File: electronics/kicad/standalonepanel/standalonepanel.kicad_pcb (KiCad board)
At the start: 2 copper layers, 135 x 54 mm, 87 parts, among them J1 Speaker, J2 POWER, P1 USB-C, P2 USB-A, SW1 TST-ESP32, SW2 BOOT, SW3 TST-ICE40, SW4 RESET, U1 SC189ZSKTRT, U10 MPU-6050, U2 SC189CSKTRT, U3 ESP32-WROVER-E, U4 CH340C, U5 MAX3421E, U6 IS64WV25616EFBLL-10TLI, U7 ICE40-HX4K, U8 DS3231, U9 MAX98357A, X2 12MHz

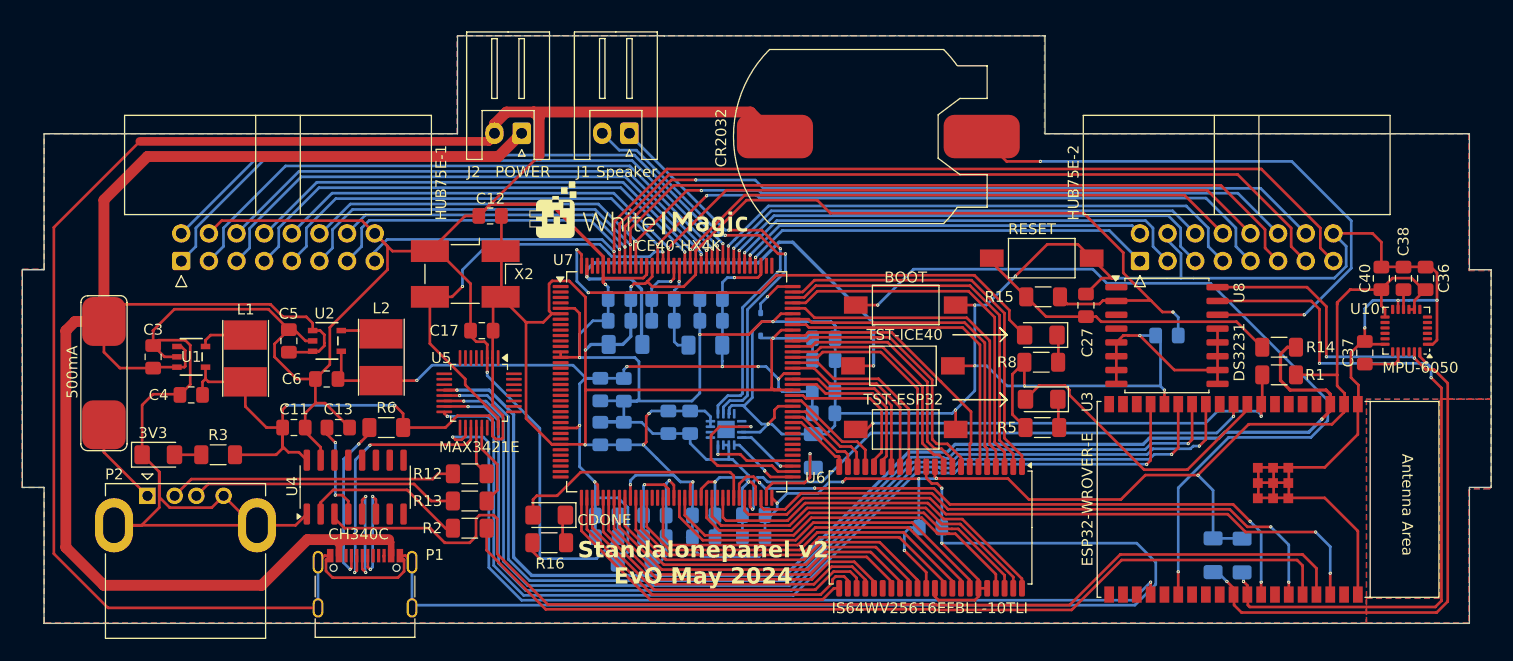
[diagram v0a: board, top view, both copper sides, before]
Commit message: Schematic v2 PCB version v2 send for production
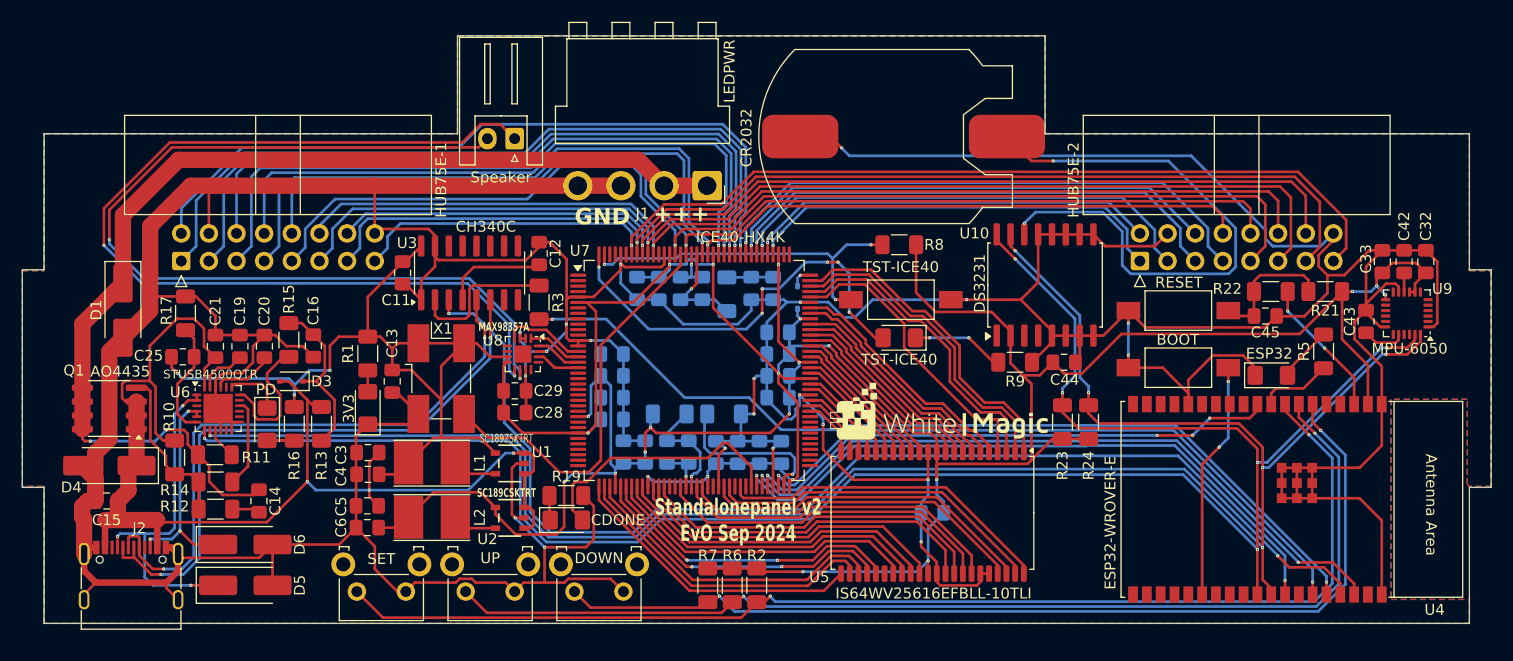
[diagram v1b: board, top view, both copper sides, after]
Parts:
- removed F1: 500mA, 0_project:FUSEHOLDER 1808
- removed P1: USB-C, 0_project:USB_C_Receptacle_G-Switch_GT-USB-7010ASV
- removed P2: USB-A, 0_project:USB-A TH Female
- removed X2: 12MHz, 0_project:Oscillator_SMD_EuroQuartz_XO91-4Pin_7.0x5.0mm_HandSoldering
- added C39: 100nF, Capacitor_SMD:C_0805_2012Metric_Pad1.18x1.45mm_HandSolder, B.Cu at (101.2, 128.2)
- added C41: 4.7uF, Capacitor_SMD:C_0805_2012Metric_Pad1.18x1.45mm_HandSolder, B.Cu at (105.2, 128.2)
- added C42: 100nF, Capacitor_SMD:C_0805_2012Metric_Pad1.18x1.45mm_HandSolder, F.Cu at (171.0, 110.8)
- added C43: 2.2nF/50V, Capacitor_SMD:C_0805_2012Metric_Pad1.18x1.45mm_HandSolder, F.Cu at (167.5, 116.2)
- added C44: 100nF, Capacitor_SMD:C_0805_2012Metric_Pad1.18x1.45mm_HandSolder, F.Cu at (139.8, 120.0)
- added C45: 100nF, Capacitor_SMD:C_0805_2012Metric_Pad1.18x1.45mm_HandSolder, F.Cu at (158.2, 115.8)
- added D1: P4SMA27A, Diode_SMD:D_SMA_Handsoldering, F.Cu at (53.2, 115.2)
- added D3: BAT760, Diode_SMD:D_SOD-323, F.Cu at (68.8, 121.8)
- added D4: P4SMA27A, Diode_SMD:D_SMA_Handsoldering, F.Cu at (52.0, 129.5)
- added D5: P4SMA27A, Diode_SMD:D_SMA_Handsoldering, F.Cu at (64.5, 140.5)
- added D6: P4SMA27A, Diode_SMD:D_SMA_Handsoldering, F.Cu at (64.5, 136.8)
- added J3: Speaker, Connector_JST:JST_XH_S2B-XH-A_1x02_P2.50mm_Horizontal, F.Cu at (89.2, 99.5)
- added LED5: CDONE, LED_SMD:LED_1206_3216Metric_Pad1.42x1.75mm_HandSolder, F.Cu at (94.0, 134.5)
- added Q1: AO4435, Package_SO:SOIC-8_3.9x4.9mm_P1.27mm, F.Cu at (52.0, 124.2)
- added R18: 10K, Resistor_SMD:R_1206_3216Metric_Pad1.30x1.75mm_HandSolder, B.Cu at (108.5, 124.8)
- added R19: 22R, Resistor_SMD:R_1206_3216Metric_Pad1.30x1.75mm_HandSolder, F.Cu at (94.0, 132.2)
- added R20: 100R, Resistor_SMD:R_1206_3216Metric_Pad1.30x1.75mm_HandSolder, B.Cu at (103.5, 124.8)
- added R21: 10K, Resistor_SMD:R_1206_3216Metric_Pad1.30x1.75mm_HandSolder, F.Cu at (163.8, 113.5)
- added R22: 100R, Resistor_SMD:R_1206_3216Metric_Pad1.30x1.75mm_HandSolder, F.Cu at (158.8, 113.5)
- added R23: 2K7, Resistor_SMD:R_1206_3216Metric_Pad1.30x1.75mm_HandSolder, F.Cu at (139.6, 125.5)
- added R24: 2K7, Resistor_SMD:R_1206_3216Metric_Pad1.30x1.75mm_HandSolder, F.Cu at (142.0, 125.5)
- added SW5: TST-ICE40, Button_Switch_SMD:SW_SPST_FSMSM, F.Cu at (124.8, 114.2)
- added SW6: RESET, Button_Switch_SMD:SW_SPST_FSMSM, F.Cu at (150.2, 115.2)
- added X1: 12MHz, 0_project:Oscillator_SMD_EuroQuartz_XO91-4Pin_7.0x5.0mm_HandSoldering, F.Cu at (82.5, 121.5)
- C14, C25, C29, C33, R7: moved to F.Cu
- C15, C20: value 100nF -> 1uF; moved to F.Cu
- C16, C19, C21: value 4.7uF -> 1uF; moved to F.Cu
- C17: value 1uF -> 100nF; moved to B.Cu
- C18, C31, C34: value 100nF -> 4.7uF
- C23: value 10uF -> 4.7uF
- C27, C40: moved to B.Cu
- C28: value 4.7uF -> 10uF; moved to F.Cu
- C30, C35: value 4.7uF -> 100nF
- C32: value 4.7uF -> 10nF; moved to F.Cu
- C36: value 10nF -> 4.7uF; moved to B.Cu
- C37: value 2.2nF/50V -> 100nF; moved to B.Cu
- C38: value 100nF -> 4.7uF; moved to B.Cu
- J1: value Speaker -> LEDPWR; footprint Connector_JST:JST_XH_S2B-XH-A_1x02_P2.50mm_Horizontal -> 0_project:JST_VH_1x04_P3.96mm_Horizontal
- J2: value POWER -> USB_C-PD; footprint Connector_JST:JST_XH_S2B-XH-A_1x02_P2.50mm_Horizontal -> 0_project:USB_C_Receptacle_G-Switch_GT-USB-7010ASV
- LED1: value ESP32 -> 3V3
- LED2: value 3V3 -> ESP32
- LED4: value CDONE -> PD
- R1: value 10K -> 1K5
- R10: value 2K7 -> 100K; moved to F.Cu
- R11: value 2K7 -> 1K; moved to F.Cu
- R12: value 33R -> 100R
- R13: value 33R -> 470R
- R14: value 100R -> 22K
- R15: value 10K -> 1K
- R16: value 22R -> 1K5
- R17: value 100R -> 10K; moved to F.Cu
- R2: value 47R -> 10K
- R3: value 1K5 -> 47R
- R6: value 5K1 -> 10K
- R8: value 2K2 -> 10K
- R9: value 10K -> 2K2; moved to F.Cu
- SW1: value TST-ESP32 -> SET; footprint Button_Switch_SMD:SW_SPST_FSMSM -> 0_project:SW_Tactile_SKHH_Angled
- SW3: value TST-ICE40 -> UP; footprint Button_Switch_SMD:SW_SPST_FSMSM -> 0_project:SW_Tactile_SKHH_Angled
- SW4: value RESET -> DOWN; footprint Button_Switch_SMD:SW_SPST_FSMSM -> 0_project:SW_Tactile_SKHH_Angled
- U10: value MPU-6050 -> DS3231; footprint 0_project:InvenSense_QFN-24_4x4mm_P0.5mm -> Package_SO:SOIC-16W_7.5x10.3mm_P1.27mm
- U3: value ESP32-WROVER-E -> CH340C; footprint 0_project:ESP32-WROVER-E -> Package_SO:SOIC-16_3.9x9.9mm_P1.27mm
- U4: value CH340C -> ESP32-WROVER-E; footprint Package_SO:SOIC-16_3.9x9.9mm_P1.27mm -> 0_project:ESP32-WROVER-E
- U5: value MAX3421E -> IS64WV25616EFBLL-10TLI; footprint 0_project:PQFP-32_5x5mm_P0.5mm -> Package_SO:TSOP-II-44_10.16x18.41mm_P0.8mm
- U6: value IS64WV25616EFBLL-10TLI -> STUSB4500QTR; footprint Package_SO:TSOP-II-44_10.16x18.41mm_P0.8mm -> 0_project:QFN-24-1EP_4x4mm_P0.5mm_EP2.7x2.7mm
- U8: value DS3231 -> MAX98357A; footprint Package_SO:SOIC-16W_7.5x10.3mm_P1.27mm -> Package_DFN_QFN:TQFN-16-1EP_3x3mm_P0.5mm_EP1.6x1.6mm
- U9: value MAX98357A -> MPU-6050; footprint Package_DFN_QFN:TQFN-16-1EP_3x3mm_P0.5mm_EP1.6x1.6mm -> 0_project:InvenSense_QFN-24_4x4mm_P0.5mm; moved to F.Cu
- moved LED2 102.6 mm to (158.8, 121.2)
- moved R14 98.5 mm to (61.8, 131.0), turned to 0 degrees
- moved R10 95.9 mm to (58.0, 128.8)
- moved R11 94.9 mm to (61.7, 128.5), turned to 0 degrees
- moved U4 86.1 mm to (160.7, 132.6), turned to -90 degrees
- moved C14 84.8 mm to (65.8, 132.8), turned to -90 degrees
- moved R1 83.8 mm to (75.8, 119.2), turned to 90 degrees
- moved U3 76.3 mm to (85.1, 111.8), turned to 90 degrees
- moved C38 73.4 mm to (99.2, 128.2)
- moved C32 70.4 mm to (173.0, 110.8), turned to -90 degrees
- moved R15 69.4 mm to (68.5, 117.9), turned to -90 degrees
- moved C40 67.6 mm to (103.2, 128.2)
- moved C33 67.3 mm to (169.0, 110.8), turned to -90 degrees
- moved C15 67.2 mm to (51.8, 132.8), turned to 180 degrees
- moved U6 66.4 mm to (62.0, 124.2), turned to 0 degrees
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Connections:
- C12 pad 1: +3V3 -> Net-(U3-V3)
- C13 pad 1: Net-(U4-V3) -> +3V3
- C14 pad 1: GND -> VPANEL
- C14 pad 2: +3V3 -> Net-(C14-Pad2)
- C15 pad 1: +3V3 -> VBUS
- C16 pad 1: +3V3 -> Net-(D3-K)
- C17 pad 1: GND -> +3V3
- C17 pad 2: +3V3 -> GND
- C18 pad 1: +1V2 -> +3V3
- C19 pad 1: +1V2 -> Net-(U6-VREG_2V7)
- C20 pad 1: +3V3 -> Net-(U6-VREG_1V2)
- C21 pad 1: GND -> VBUS
- C21 pad 2: +1V2 -> GND
- C22 pad 1: GND -> +1V2
- C22 pad 2: +1V2 -> GND
- C23 pad 1: +3V3 -> +1V2
- C25 pad 2: GND -> Net-(U6-RESET)
- C26 pad 1: +3V3 -> GND
- C26 pad 2: GND -> +1V2
- C27 pad 1: Net-(C27-Pad1) -> GND
- C27 pad 2: GND -> +1V2
- C28 pad 1: GND -> +3V3
- C28 pad 2: +1V2 -> GND
- C29 pad 1: GND -> +3V3
- C29 pad 2: +1V2 -> GND
- C3 pad 1: +5V -> VBUS
- C30 pad 1: GND -> +3V3
- C30 pad 2: +3V3 -> GND
- C31 pad 1: GND -> +3V3
- C31 pad 2: +3V3 -> GND
- C34 pad 1: Net-(U7-VCCPLL0) -> GND
- C34 pad 2: Net-(U7-GNDPLL0) -> +3V3
- C35 pad 1: Net-(U7-VCCPLL0) -> GND
- C35 pad 2: Net-(U7-GNDPLL0) -> +3V3
- C37 pad 2: Net-(U10-CPOUT) -> +3V3
- C38 pad 2: Net-(U10-REGOUT) -> +1V2
- C40 pad 1: GND -> Net-(U7-VCCPLL0)
- C40 pad 2: +3V3 -> Net-(U7-GNDPLL0)
- C5 pad 1: +5V -> VBUS
- J1 pad 1: Net-(J1-Pin_1) -> VPANEL
- J1 pad 2: Net-(J1-Pin_2) -> VPANEL
- LED1 pad 1: Net-(LED1-K) -> GND
- R1 pad 1: +3V3 -> Net-(LED1-A)
- R1 pad 2: Net-(U3-32K_XP/GPIO32/ADC1_CH4) -> +3V3
- R10 pad 1: +3V3 -> VBUS
- R10 pad 2: I2C-CLK -> Net-(Q1-G1)
- R11 pad 1: +3V3 -> VPANEL
- R11 pad 2: I2C-SDA -> Net-(U6-DISCH)
- R12 pad 1: Net-(P2-D-) -> Net-(C14-Pad2)
- R12 pad 2: Net-(U5-D-) -> Net-(Q1-G1)
- R13 pad 1: Net-(P2-D+) -> VBUS
- R13 pad 2: Net-(U5-D+) -> Net-(D3-K)
- R14 pad 1: ~{RESET} -> Net-(Q1-G1)
- R14 pad 2: Net-(C27-Pad1) -> Net-(U6-VBUS_EN_SNK)
- R15 pad 1: +3V3 -> Net-(D3-K)
- R15 pad 2: Net-(C27-Pad1) -> Net-(U6-VBUS_VS_DISCH)
- R16 pad 1: Net-(LED4-K) -> Net-(LED4-A)
- R16 pad 2: GND -> +3V3
- R17 pad 1: Net-(U7-VCCPLL0) -> Net-(U6-RESET)
- R17 pad 2: +1V2 -> GND
- R2 pad 1: Net-(U3-U0RXD/GPIO3) -> +3V3
- R2 pad 2: Net-(U4-TXD) -> Net-(U4-32K_XP/GPIO32/ADC1_CH4)
- R3 pad 1: Net-(LED2-A) -> Net-(U4-U0RXD/GPIO3)
- R3 pad 2: +3V3 -> Net-(U3-TXD)
- R5 pad 1: Net-(LED1-K) -> Net-(U4-32K_XN/GPIO33/ADC1_CH5)
- R5 pad 2: GND -> Net-(LED2-A)
- R6 pad 1: Net-(P1-CC) -> +3V3
- R6 pad 2: +3V3 -> Net-(U4-GPIO35/ADC1_CH7)
- R7 pad 2: Net-(U7-IOT_221) -> Net-(U4-GPIO34/ADC1_CH6)
- R8 pad 1: Net-(LED3-K) -> +3V3
- R8 pad 2: GND -> Net-(U7-IOT_221)
- R9 pad 1: Net-(U7-IOB_108_SS) -> Net-(LED3-K)
- SW1 pad 2: Net-(U3-32K_XP/GPIO32/ADC1_CH4) -> Net-(U4-32K_XP/GPIO32/ADC1_CH4)
- SW2 pad 1: Net-(U3-GPIO0/BOOT/ADC2_CH1) -> Net-(U4-GPIO0/BOOT/ADC2_CH1)
- SW3 pad 2: Net-(U7-IOT_221) -> Net-(U4-GPIO35/ADC1_CH7)
- SW4 pad 2: Net-(C27-Pad1) -> Net-(U4-GPIO34/ADC1_CH6)
- U1 pad 1: +5V -> VBUS
- U1 pad 3: +5V -> VBUS
- U10 pad 1: GND -> unconnected-(U10-32KHZ-Pad1)
- U10 pad 10: Net-(U10-REGOUT) -> GND
- U10 pad 12: unconnected-(U10-INT-Pad12) -> GND
- U10 pad 13: +3V3 -> GND
- U10 pad 14: unconnected-(U10-NC-Pad14) -> Net-(BT1-+)
- U10 pad 15: unconnected-(U10-NC-Pad15) -> I2C-SDA
- U10 pad 16: unconnected-(U10-NC-Pad16) -> I2C-CLK
- U10 pad 2: unconnected-(U10-NC-Pad2) -> +3V3
- U10 pad 5: unconnected-(U10-NC-Pad5) -> GND
- U10 pad 6: unconnected-(U10-AUX_DA-Pad6) -> GND
- U10 pad 7: unconnected-(U10-AUX_CL-Pad7) -> GND
- U10 pad 8: +3V3 -> GND
- U10 pad 9: +3V3 -> GND
- U2 pad 1: +5V -> VBUS
- U2 pad 3: +5V -> VBUS
- U3 pad 10: VSPI-SDI -> unconnected-(U3-~{DSR}-Pad10)
- U3 pad 12: HSPI-CS-USB -> unconnected-(U3-~{DCD}-Pad12)
- U3 pad 13: HSPI-CLK -> unconnected-(U3-~{DTR}-Pad13)
- U3 pad 14: HSPI-SDO -> unconnected-(U3-~{RTS}-Pad14)
- U3 pad 16: HSPI-SDI -> +3V3
- U3 pad 2: +3V3 -> Net-(U3-TXD)
- U3 pad 3: ~{RESET} -> Net-(U3-RXD)
- U3 pad 4: unconnected-(U3-SENSOR_VP/GPIO36/ADC1_CH0-Pad4) -> Net-(U3-V3)
- U3 pad 5: unconnected-(U3-SENSOR_VN/GPIO39/ADC1_CH3-Pad5) -> Net-(U3-UD+)
- U3 pad 6: unconnected-(U3-GPIO34/ADC1_CH6-Pad6) -> Net-(U3-UD-)
- U3 pad 8: Net-(U3-32K_XP/GPIO32/ADC1_CH4) -> unconnected-(U3-NC-Pad8)
- U3 pad 9: Net-(LED1-A) -> unconnected-(U3-~{CTS}-Pad9)
- U4 pad 10: unconnected-(U4-~{DSR}-Pad10) -> VSPI-SDI
- U4 pad 16: +3V3 -> unconnected-(U4-MTCK/GPIO13/ADC2_CH4-Pad16)
- U4 pad 2: Net-(U4-TXD) -> +3V3
- U4 pad 3: Net-(U3-U0TXD/GPIO1) -> ~{RESET}
- U4 pad 4: Net-(U4-V3) -> unconnected-(U4-SENSOR_VP/GPIO36/ADC1_CH0-Pad4)
- U4 pad 5: Net-(P1-D+) -> unconnected-(U4-SENSOR_VN/GPIO39/ADC1_CH3-Pad5)
- U4 pad 6: Net-(P1-D-) -> Net-(U4-GPIO34/ADC1_CH6)
- U4 pad 7: unconnected-(U4-NC-Pad7) -> Net-(U4-GPIO35/ADC1_CH7)
- U4 pad 8: unconnected-(U4-NC-Pad8) -> Net-(U4-32K_XP/GPIO32/ADC1_CH4)
- U4 pad 9: unconnected-(U4-~{CTS}-Pad9) -> Net-(U4-32K_XN/GPIO33/ADC1_CH5)
- U5 pad 1: unconnected-(U5-GPIN7-Pad1) -> RAM-A0
- U5 pad 10: unconnected-(U5-GPOUT6-Pad10) -> RAM-D3
- U5 pad 11: unconnected-(U5-GPOUT7-Pad11) -> +3V3
- U5 pad 12: ~{RESET} -> GND
- U5 pad 13: HSPI-CLK -> RAM-D4
- U5 pad 14: HSPI-CS-USB -> RAM-D5
- U5 pad 15: HSPI-SDO -> RAM-D6
- U5 pad 16: HSPI-SDI -> RAM-D7
- U5 pad 17: unconnected-(U5-GPX-Pad17) -> RAM-WE
- U5 pad 18: HSPI-INT -> RAM-A5
- U5 pad 19: (no net) -> RAM-A6
- U5 pad 2: +3V3 -> RAM-A1
- U5 pad 20: Net-(U5-D-) -> RAM-A7
- U5 pad 21: Net-(U5-D+) -> RAM-A8
- U5 pad 22: unconnected-(U5-VBCOMP-Pad22) -> RAM-A9
- U5 pad 23: +3V3 -> RAM-A10
- U5 pad 24: SYSCLK -> RAM-A11
- U5 pad 25: unconnected-(U5-XO-Pad25) -> RAM-A12
- U5 pad 26: unconnected-(U5-GPIN0-Pad26) -> RAM-A13
- U5 pad 27: unconnected-(U5-GPIN1-Pad27) -> RAM-A14
- U5 pad 29: unconnected-(U5-GPIN3-Pad29) -> RAM-D8
- U5 pad 3: GND -> RAM-A2
- U5 pad 30: unconnected-(U5-GPIN4-Pad30) -> RAM-D9
- U5 pad 31: unconnected-(U5-GPIN5-Pad31) -> RAM-D10
- U5 pad 32: unconnected-(U5-GPIN6-Pad32) -> RAM-D11
- U5 pad 4: unconnected-(U5-GPOUT0-Pad4) -> RAM-A3
- U5 pad 5: unconnected-(U5-GPOUT1-Pad5) -> RAM-A4
- U5 pad 6: unconnected-(U5-GPOUT2-Pad6) -> RAM-CS
- U5 pad 7: unconnected-(U5-GPOUT3-Pad7) -> RAM-D0
- U5 pad 8: unconnected-(U5-GPOUT4-Pad8) -> RAM-D1
- U5 pad 9: unconnected-(U5-GPOUT5-Pad9) -> RAM-D2
- U6 pad 1: RAM-A0 -> Net-(D5-K)
- U6 pad 10: RAM-D3 -> GND
- U6 pad 11: +3V3 -> unconnected-(U6-ATTACH-Pad11)
- U6 pad 13: RAM-D4 -> GND
- U6 pad 14: RAM-D5 -> unconnected-(U6-POWER_OK3-Pad14)
- U6 pad 15: RAM-D6 -> unconnected-(U6-GPIO-Pad15)
- U6 pad 16: RAM-D7 -> Net-(U6-VBUS_EN_SNK)
- U6 pad 17: RAM-WE -> unconnected-(U6-A_B_SIDE-Pad17)
- U6 pad 18: RAM-A5 -> Net-(U6-VBUS_VS_DISCH)
- U6 pad 19: RAM-A6 -> Net-(LED4-K)
- U6 pad 2: RAM-A1 -> Net-(D5-K)
- U6 pad 20: RAM-A7 -> unconnected-(U6-POWER_OK2-Pad20)
- U6 pad 21: RAM-A8 -> Net-(U6-VREG_1V2)
- U6 pad 22: RAM-A9 -> GND
- U6 pad 23: RAM-A10 -> Net-(U6-VREG_2V7)
- U6 pad 24: RAM-A11 -> VBUS
- U6 pad 25: RAM-A12 -> GND
- U6 pad 3: RAM-A2 -> unconnected-(U6-NC-Pad3)
- U6 pad 4: RAM-A3 -> Net-(D6-K)
- U6 pad 5: RAM-A4 -> Net-(D6-K)
- U6 pad 6: RAM-CS -> Net-(U6-RESET)
- U6 pad 7: RAM-D0 -> I2C-CLK
- U6 pad 8: RAM-D1 -> I2C-SDA
- U6 pad 9: RAM-D2 -> Net-(U6-DISCH)
- U7 pad 15: unconnected-(U7-IOL_10A-Pad15) -> Net-(U7-IOL_10A)
- U7 pad 16: unconnected-(U7-IOL_10B-Pad16) -> Net-(U7-IOL_10B)
- U7 pad 17: unconnected-(U7-IOL_12A-Pad17) -> Net-(U7-IOL_12A)
- U7 pad 18: unconnected-(U7-IOL_12B-Pad18) -> Net-(U7-IOL_12B)
- U7 pad 65: Net-(LED4-A) -> Net-(LED5-A)
- U7 pad 73: Net-(U7-IOR_109) -> unconnected-(U7-IOR_109-Pad73)
- U7 pad 74: Net-(U7-IOR_110) -> unconnected-(U7-IOR_110-Pad74)
- U7 pad 75: Net-(U7-IOR_111) -> unconnected-(U7-IOR_111-Pad75)
- U7 pad 76: Net-(U7-IOR_112) -> unconnected-(U7-IOR_112-Pad76)
- U8 pad 1: unconnected-(U8-32KHZ-Pad1) -> Net-(U7-IOL_10B)
- U8 pad 10: GND -> Net-(J3-Pin_2)
- U8 pad 12: GND -> unconnected-(U8-NC-Pad12)
- U8 pad 13: GND -> unconnected-(U8-NC-Pad13)
- U8 pad 14: Net-(BT1-+) -> Net-(U7-IOL_12B)
- U8 pad 15: I2C-SDA -> GND
- U8 pad 16: I2C-CLK -> Net-(U7-IOL_12A)
- U8 pad 2: +3V3 -> GND
- U8 pad 3: unconnected-(U8-~{INT}/SQW-Pad3) -> GND
- U8 pad 4: unconnected-(U8-~{RST}-Pad4) -> Net-(U7-IOL_10A)
- U8 pad 5: GND -> unconnected-(U8-NC-Pad5)
- U8 pad 6: GND -> unconnected-(U8-NC-Pad6)
- U8 pad 7: GND -> +3V3
- U8 pad 8: GND -> +3V3
- U8 pad 9: GND -> Net-(J3-Pin_1)
- U9 pad 1: Net-(U7-IOR_109) -> GND
- U9 pad 10: Net-(J1-Pin_2) -> Net-(U9-REGOUT)
- U9 pad 13: unconnected-(U9-NC-Pad13) -> +3V3
- U9 pad 14: Net-(U7-IOR_110) -> unconnected-(U9-NC-Pad14)
- U9 pad 15: GND -> unconnected-(U9-NC-Pad15)
- U9 pad 16: Net-(U7-IOR_111) -> unconnected-(U9-NC-Pad16)
- U9 pad 17: (no net) -> unconnected-(U9-NC-Pad17)
- U9 pad 2: GND -> unconnected-(U9-NC-Pad2)
- U9 pad 3: GND -> unconnected-(U9-NC-Pad3)
- U9 pad 4: Net-(U7-IOR_112) -> unconnected-(U9-NC-Pad4)
- U9 pad 7: +3V3 -> unconnected-(U9-AUX_CL-Pad7)
- U9 pad 9: Net-(J1-Pin_1) -> +3V3
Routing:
- net GND: track 835.5 -> 664.8 mm, vias 22 -> 21
- net +5V: track 153.1 -> 0.00 mm
- net VBUS: track 0.00 -> 114.7 mm, vias 0 -> 3
- net I2C-SDA: track 69.6 -> 180.7 mm, vias 4 -> 6
- net Net-(U4-32K_XP/GPIO32/ADC1_CH4): track 0.00 -> 110.7 mm, vias 0 -> 2
- net I2C-CLK: track 72.6 -> 182.5 mm, vias 3 -> 6
- net Net-(U3-RXD): track 0.00 -> 107.9 mm, vias 0 -> 2
- net Net-(U3-U0TXD/GPIO1): track 103.8 -> 0.00 mm
- net Net-(U4-GPIO35/ADC1_CH7): track 0.00 -> 101.0 mm, vias 0 -> 2
- net ~{RESET}: track 113.4 -> 12.9 mm
- net VPANEL: track 0.00 -> 99.7 mm, vias 0 -> 2
- net HSPI-CS-USB: track 93.6 -> 0.00 mm, vias 2 -> 0
- net HSPI-CLK: track 92.2 -> 0.00 mm, vias 2 -> 0
- net HSPI-SDO: track 91.7 -> 0.00 mm, vias 2 -> 0
- net Net-(U4-GPIO34/ADC1_CH6): track 0.00 -> 91.3 mm, vias 0 -> 2
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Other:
- board text added: "+++"
- board text added: "GND"
- board text added: "Standalonepanel v2 EvO Sep 2024"
- board text removed: "Standalonepanel v2 EvO May 2024"
